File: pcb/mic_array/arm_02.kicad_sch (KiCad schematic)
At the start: 16 parts, among them U17 IM72D128V01XTMA1, U18 IM72D128V01XTMA1, U19 IM72D128V01XTMA1, U20 IM72D128V01XTMA1, U21 IM72D128V01XTMA1, U22 IM72D128V01XTMA1, U23 IM72D128V01XTMA1, U24 IM72D128V01XTMA1

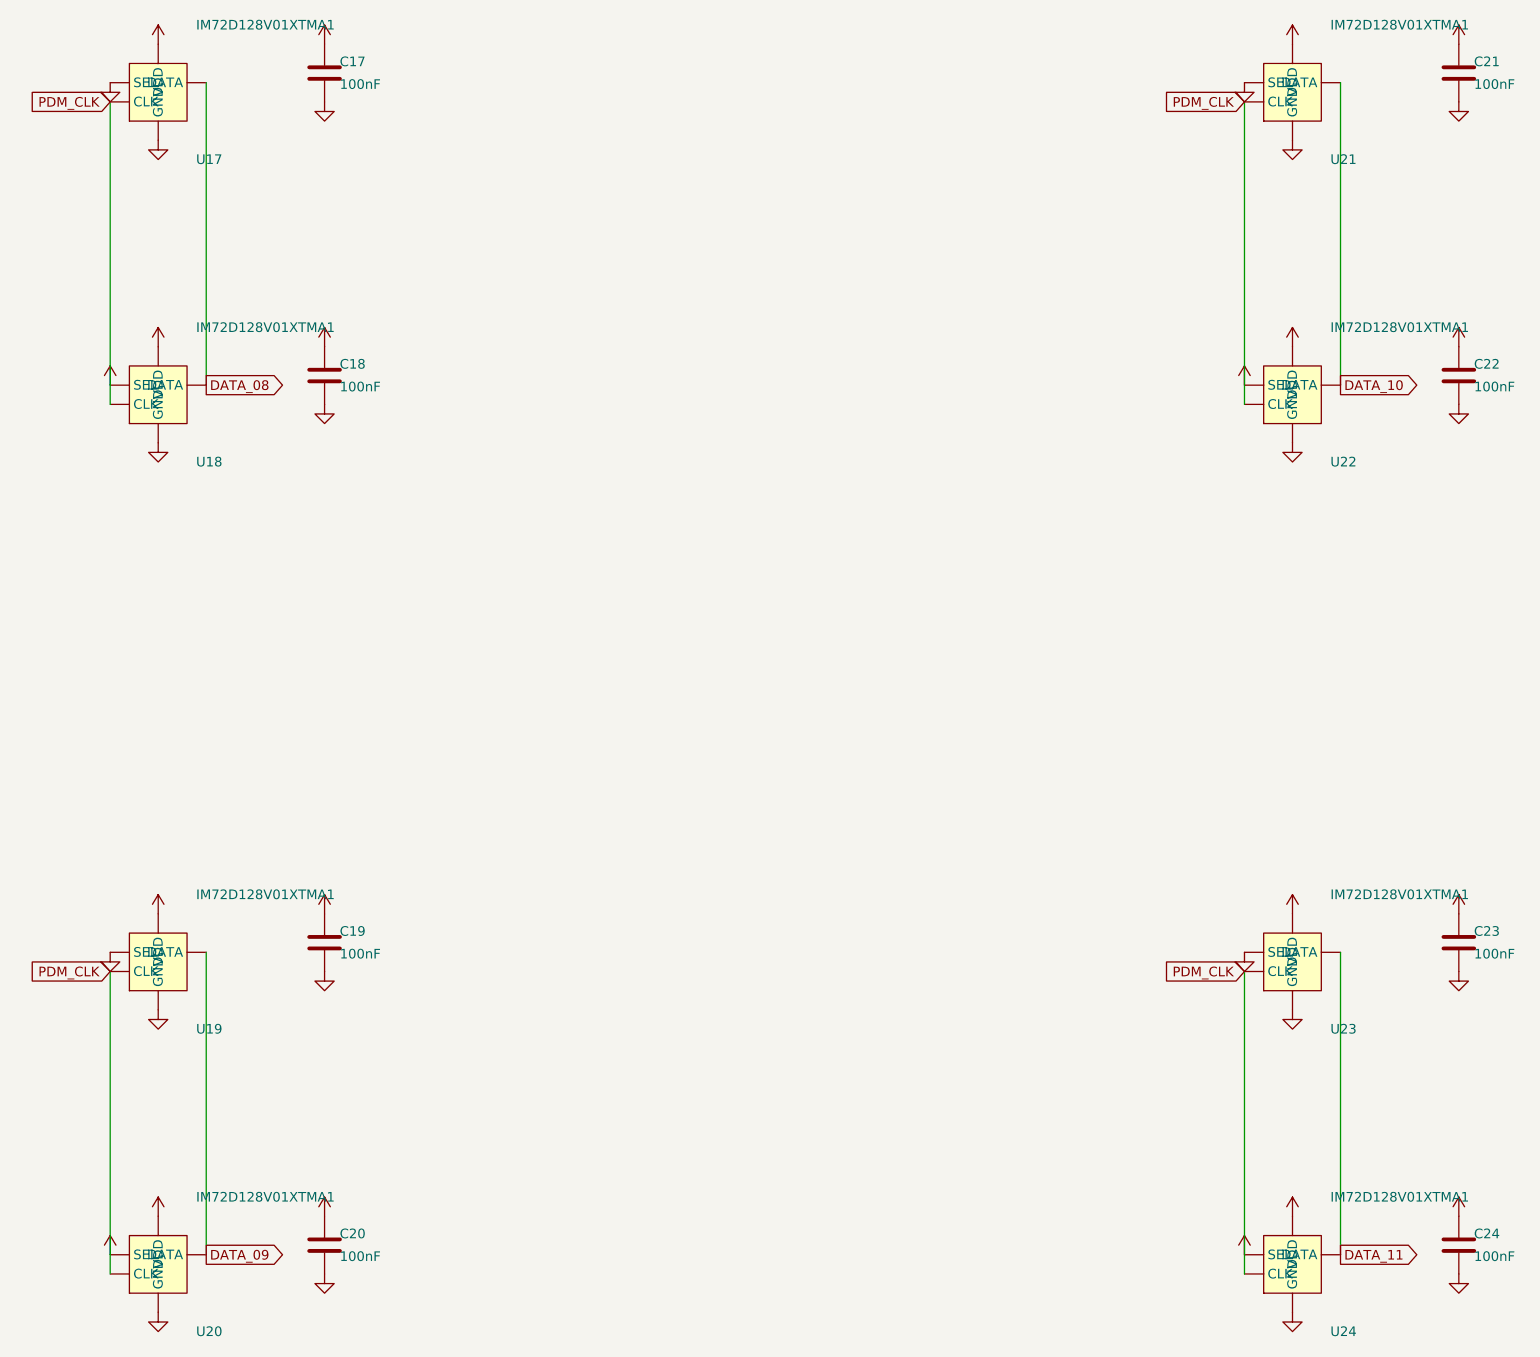
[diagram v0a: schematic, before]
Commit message: Updated.
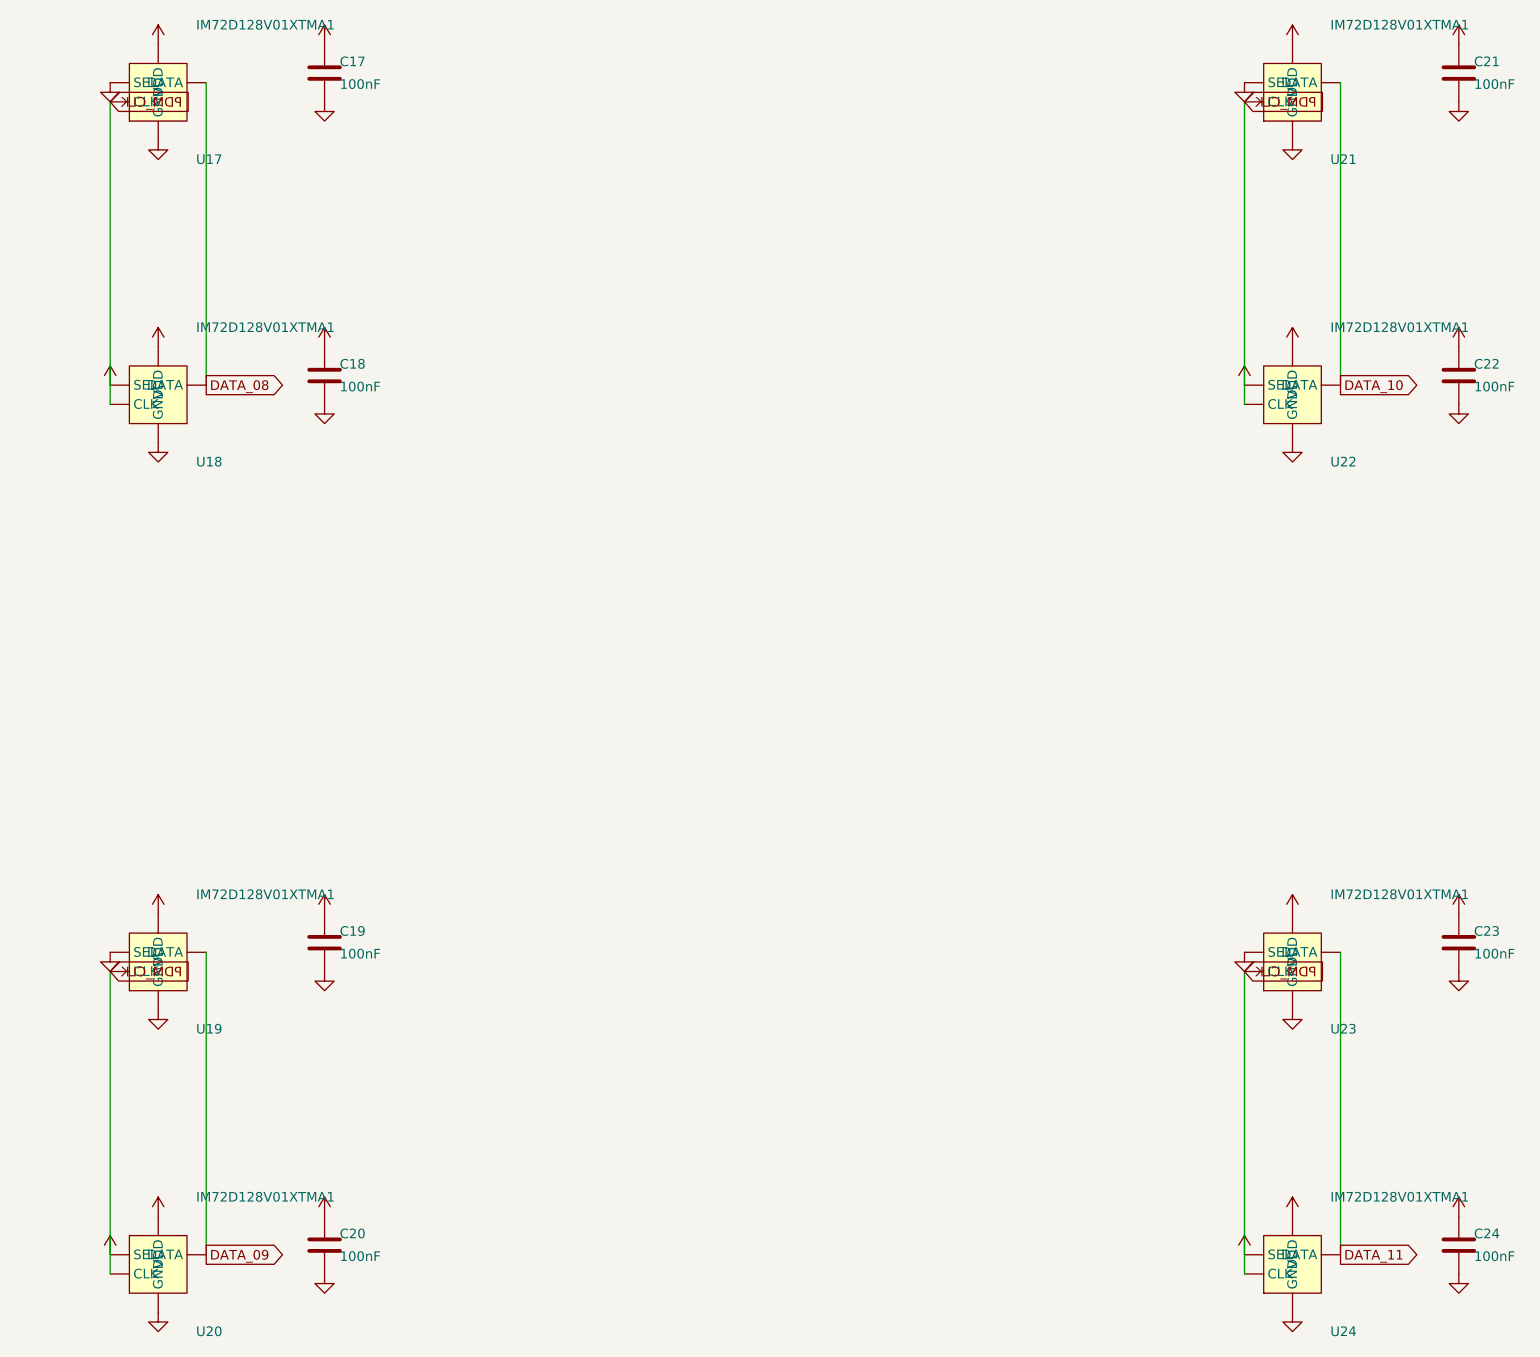
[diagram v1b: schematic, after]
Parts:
- C17, C18, C19, C20, C21, C22, C23, C24: footprint Capacitor_SMD:C_0402_1005Metric -> (none)
- U17, U18, U19, U20, U21, U22, U23, U24: footprint Sensor_Audio:Infineon_PG-LLGA-5-2 -> (none)
